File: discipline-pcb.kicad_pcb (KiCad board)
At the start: 2 copper layers, 357.2 x 120.3 mm, 160 parts, among them SW1 KEYSW, SW10 KEYSW, SW11 KEYSW, SW12 KEYSW, SW13 KEYSW, SW14 KEYSW, SW16 KEYSW, SW17 KEYSW, SW18 KEYSW, SW19 KEYSW, SW2 KEYSW, SW20 KEYSW, SW21 KEYSW, SW22 KEYSW, SW23 KEYSW, SW24 KEYSW, SW25 KEYSW, SW26 KEYSW, SW27 KEYSW, SW28 KEYSW, SW29 KEYSW, SW3 KEYSW, SW31 KEYSW, SW32 KEYSW, SW33 KEYSW, SW34 KEYSW, SW35 KEYSW, SW36 KEYSW, SW37 KEYSW, SW38 KEYSW, SW39 KEYSW, SW4 KEYSW, SW40 KEYSW, SW41 KEYSW, SW42 KEYSW, SW43 KEYSW, SW45 KEYSW, SW46 KEYSW, SW47 KEYSW, SW48 KEYSW, SW49 KEYSW, SW5 KEYSW, SW50 KEYSW, SW51 KEYSW, SW52 KEYSW, SW53 KEYSW, SW54 KEYSW, SW55 KEYSW, SW56 KEYSW, SW57 KEYSW, SW59 KEYSW, SW6 KEYSW, SW60 KEYSW, SW61 KEYSW, SW62 KEYSW, SW7 KEYSW, SW72 KEYSW, SW73 KEYSW, SW74 KEYSW, SW75 KEYSW, SW76 KEYSW, SW77 KEYSW, SW78 KEYSW, SW79 KEYSW, SW8 KEYSW, SW80 KEYSW, SW81 KEYSW, SW82 KEYSW, SW83 KEYSW, SW9 KEYSW

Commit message: update to hotswap; needs rerouting
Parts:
- removed ST62: 7U, cftkb:MX-7U-Stabilizer
- SW1, SW10, SW11, SW12, SW13, SW17, SW18, SW19, SW2, SW20, SW21, SW22, SW23, SW24, SW25, SW26, SW27, SW28, SW3, SW32, SW33, SW34, SW35, SW36, SW37, SW38, SW39, SW4, SW40, SW41, SW42, SW46, SW47, SW48, SW49, SW5, SW50, SW51, SW52, SW53, SW54, SW55, SW6, SW7, SW72, SW75, SW76, SW77, SW78, SW79, SW8, SW80, SW81, SW82, SW83, SW9: footprint cftkb:SW_Cherry_MX1A_1.00u_PCB-NOSCREEN -> MX_Hotswap:MX-Hotswap-1U; moved to B.Cu
- SW14: footprint cftkb:SW_Cherry_MX1A_2.00u_PCBNOSCREEN -> MX_Hotswap:MX-Hotswap-2U; moved to B.Cu
- SW16, SW29, SW73, SW74: footprint cftkb:SW_Cherry_MX1A_1.50u_PCBNOSCREEN -> MX_Hotswap:MX-Hotswap-1.5U; moved to B.Cu
- SW31: footprint cftkb:SW_Cherry_MX1A_1.75u_PCBNOSCREEN -> MX_Hotswap:MX-Hotswap-1.75U; moved to B.Cu
- SW43, SW45: footprint cftkb:SW_Cherry_MX1A_2.25u_PCBNOSCREEN -> MX_Hotswap:MX-Hotswap-2.25U; moved to B.Cu
- SW56: footprint cftkb:SW_Cherry_MX1A_2.75u_PCB_NOSCREEN -> MX_Hotswap:MX-Hotswap-2.75U; moved to B.Cu
- SW57, SW59, SW60, SW61: footprint cftkb:SW_Cherry_MX1A_1.25u_PCBNOSCREEN -> MX_Hotswap:MX-Hotswap-1.25U; moved to B.Cu
- SW62: footprint cftkb:SW_Cherry_MX1A_1.00u_PCB-NOSCREEN -> MX_Hotswap:MX-Hotswap-7U-ReversedStabilizers; moved to B.Cu
- moved ? 20.6 mm to (399.5, 104.5)
- moved SW10 5.68 mm to (234.8, 94.8), turned to 180 degrees
- moved SW11 5.68 mm to (253.8, 94.8), turned to 180 degrees
- moved SW5 5.68 mm to (139.5, 94.8), turned to 180 degrees
- moved SW50 5.68 mm to (182.4, 151.9), turned to 180 degrees
- moved SW54 5.68 mm to (258.6, 151.9), turned to 180 degrees
- moved SW55 5.68 mm to (277.7, 151.9), turned to 180 degrees
- moved SW56 5.68 mm to (313.4, 151.9), turned to 180 degrees
- moved SW75 5.68 mm to (382.4, 94.8), turned to 180 degrees
- moved SW77 5.68 mm to (382.4, 151.9), turned to 180 degrees
- moved SW79 5.68 mm to (401.5, 94.8), turned to 180 degrees
- moved SW2 5.68 mm to (82.4, 94.8), turned to 180 degrees
- moved SW3 5.68 mm to (101.4, 94.8), turned to 180 degrees
- moved SW4 5.68 mm to (120.5, 94.8), turned to 180 degrees
- moved SW45 5.68 mm to (75.2, 151.9), turned to 180 degrees
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
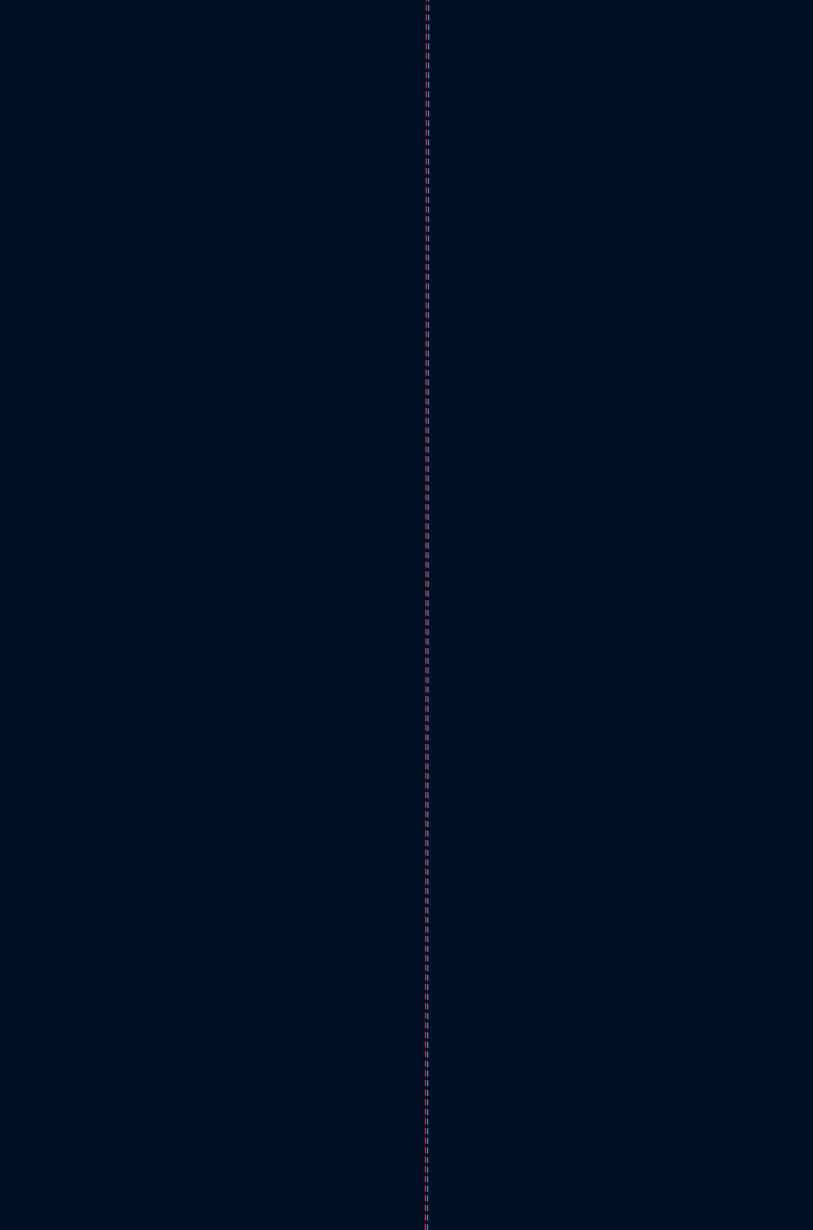
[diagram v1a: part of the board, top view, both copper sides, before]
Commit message: add leds to pcb
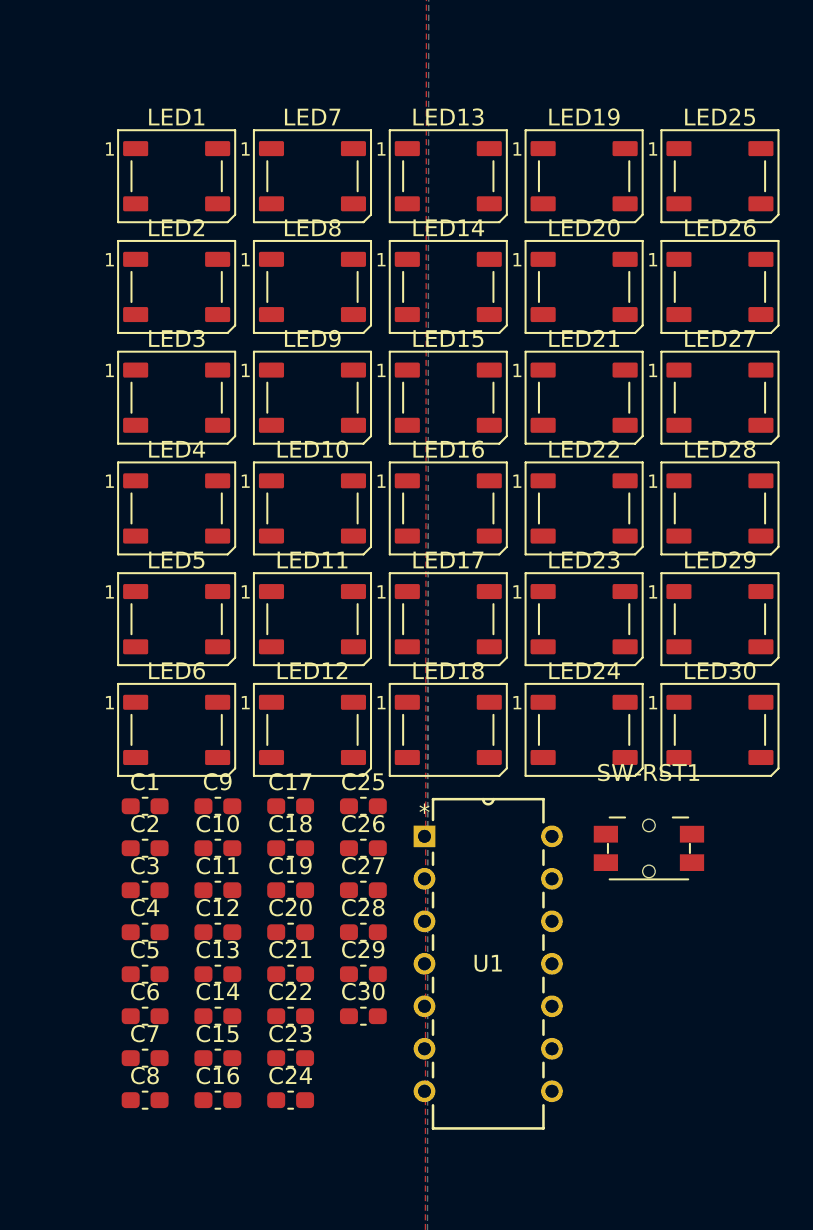
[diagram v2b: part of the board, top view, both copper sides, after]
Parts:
- added C1: 100nF 0603, Capacitor_SMD:C_0603_1608Metric_Pad1.08x0.95mm_HandSolder, F.Cu at (445.2, 128.2)
- added C10: 100nF 0603, Capacitor_SMD:C_0603_1608Metric_Pad1.08x0.95mm_HandSolder, F.Cu at (449.5, 130.7)
- added C11: 100nF 0603, Capacitor_SMD:C_0603_1608Metric_Pad1.08x0.95mm_HandSolder, F.Cu at (449.5, 133.2)
- added C12: 100nF 0603, Capacitor_SMD:C_0603_1608Metric_Pad1.08x0.95mm_HandSolder, F.Cu at (449.5, 135.7)
- added C13: 100nF 0603, Capacitor_SMD:C_0603_1608Metric_Pad1.08x0.95mm_HandSolder, F.Cu at (449.5, 138.2)
- added C14: 100nF 0603, Capacitor_SMD:C_0603_1608Metric_Pad1.08x0.95mm_HandSolder, F.Cu at (449.5, 140.7)
- added C15: 100nF 0603, Capacitor_SMD:C_0603_1608Metric_Pad1.08x0.95mm_HandSolder, F.Cu at (449.5, 143.2)
- added C16: 100nF 0603, Capacitor_SMD:C_0603_1608Metric_Pad1.08x0.95mm_HandSolder, F.Cu at (449.5, 145.7)
- added C17: 100nF 0603, Capacitor_SMD:C_0603_1608Metric_Pad1.08x0.95mm_HandSolder, F.Cu at (453.9, 128.2)
- added C18: 100nF 0603, Capacitor_SMD:C_0603_1608Metric_Pad1.08x0.95mm_HandSolder, F.Cu at (453.9, 130.7)
- added C19: 100nF 0603, Capacitor_SMD:C_0603_1608Metric_Pad1.08x0.95mm_HandSolder, F.Cu at (453.9, 133.2)
- added C2: 100nF 0603, Capacitor_SMD:C_0603_1608Metric_Pad1.08x0.95mm_HandSolder, F.Cu at (445.2, 130.7)
- added C20: 100nF 0603, Capacitor_SMD:C_0603_1608Metric_Pad1.08x0.95mm_HandSolder, F.Cu at (453.9, 135.7)
- added C21: 100nF 0603, Capacitor_SMD:C_0603_1608Metric_Pad1.08x0.95mm_HandSolder, F.Cu at (453.9, 138.2)
- added C22: 100nF 0603, Capacitor_SMD:C_0603_1608Metric_Pad1.08x0.95mm_HandSolder, F.Cu at (453.9, 140.7)
- added C23: 100nF 0603, Capacitor_SMD:C_0603_1608Metric_Pad1.08x0.95mm_HandSolder, F.Cu at (453.9, 143.2)
- added C24: 100nF 0603, Capacitor_SMD:C_0603_1608Metric_Pad1.08x0.95mm_HandSolder, F.Cu at (453.9, 145.7)
- added C25: 100nF 0603, Capacitor_SMD:C_0603_1608Metric_Pad1.08x0.95mm_HandSolder, F.Cu at (458.2, 128.2)
- added C26: 100nF 0603, Capacitor_SMD:C_0603_1608Metric_Pad1.08x0.95mm_HandSolder, F.Cu at (458.2, 130.7)
- added C27: 100nF 0603, Capacitor_SMD:C_0603_1608Metric_Pad1.08x0.95mm_HandSolder, F.Cu at (458.2, 133.2)
- added C28: 100nF 0603, Capacitor_SMD:C_0603_1608Metric_Pad1.08x0.95mm_HandSolder, F.Cu at (458.2, 135.7)
- added C29: 100nF 0603, Capacitor_SMD:C_0603_1608Metric_Pad1.08x0.95mm_HandSolder, F.Cu at (458.2, 138.2)
- added C3: 100nF 0603, Capacitor_SMD:C_0603_1608Metric_Pad1.08x0.95mm_HandSolder, F.Cu at (445.2, 133.2)
- added C30: 100nF 0603, Capacitor_SMD:C_0603_1608Metric_Pad1.08x0.95mm_HandSolder, F.Cu at (458.2, 140.7)
- added C4: 100nF 0603, Capacitor_SMD:C_0603_1608Metric_Pad1.08x0.95mm_HandSolder, F.Cu at (445.2, 135.7)
- added C5: 100nF 0603, Capacitor_SMD:C_0603_1608Metric_Pad1.08x0.95mm_HandSolder, F.Cu at (445.2, 138.2)
- added C6: 100nF 0603, Capacitor_SMD:C_0603_1608Metric_Pad1.08x0.95mm_HandSolder, F.Cu at (445.2, 140.7)
- added C7: 100nF 0603, Capacitor_SMD:C_0603_1608Metric_Pad1.08x0.95mm_HandSolder, F.Cu at (445.2, 143.2)
- added C8: 100nF 0603, Capacitor_SMD:C_0603_1608Metric_Pad1.08x0.95mm_HandSolder, F.Cu at (445.2, 145.7)
- added C9: 100nF 0603, Capacitor_SMD:C_0603_1608Metric_Pad1.08x0.95mm_HandSolder, F.Cu at (449.5, 128.2)
- added LED1: WS2812B, LED_SMD:LED_WS2812B_PLCC4_5.0x5.0mm_P3.2mm, F.Cu at (447.1, 90.5)
- added LED10: WS2812B, LED_SMD:LED_WS2812B_PLCC4_5.0x5.0mm_P3.2mm, F.Cu at (455.2, 110.4)
- added LED11: WS2812B, LED_SMD:LED_WS2812B_PLCC4_5.0x5.0mm_P3.2mm, F.Cu at (455.2, 117.0)
- added LED12: WS2812B, LED_SMD:LED_WS2812B_PLCC4_5.0x5.0mm_P3.2mm, F.Cu at (455.2, 123.6)
- added LED13: WS2812B, LED_SMD:LED_WS2812B_PLCC4_5.0x5.0mm_P3.2mm, F.Cu at (463.3, 90.5)
- added LED14: WS2812B, LED_SMD:LED_WS2812B_PLCC4_5.0x5.0mm_P3.2mm, F.Cu at (463.3, 97.1)
- added LED15: WS2812B, LED_SMD:LED_WS2812B_PLCC4_5.0x5.0mm_P3.2mm, F.Cu at (463.3, 103.7)
- added LED16: WS2812B, LED_SMD:LED_WS2812B_PLCC4_5.0x5.0mm_P3.2mm, F.Cu at (463.3, 110.4)
- added LED17: WS2812B, LED_SMD:LED_WS2812B_PLCC4_5.0x5.0mm_P3.2mm, F.Cu at (463.3, 117.0)
- added LED18: WS2812B, LED_SMD:LED_WS2812B_PLCC4_5.0x5.0mm_P3.2mm, F.Cu at (463.3, 123.6)
- added LED19: WS2812B, LED_SMD:LED_WS2812B_PLCC4_5.0x5.0mm_P3.2mm, F.Cu at (471.4, 90.5)
- added LED2: WS2812B, LED_SMD:LED_WS2812B_PLCC4_5.0x5.0mm_P3.2mm, F.Cu at (447.1, 97.1)
- added LED20: WS2812B, LED_SMD:LED_WS2812B_PLCC4_5.0x5.0mm_P3.2mm, F.Cu at (471.4, 97.1)
- added LED21: WS2812B, LED_SMD:LED_WS2812B_PLCC4_5.0x5.0mm_P3.2mm, F.Cu at (471.4, 103.7)
- added LED22: WS2812B, LED_SMD:LED_WS2812B_PLCC4_5.0x5.0mm_P3.2mm, F.Cu at (471.4, 110.4)
- added LED23: WS2812B, LED_SMD:LED_WS2812B_PLCC4_5.0x5.0mm_P3.2mm, F.Cu at (471.4, 117.0)
- added LED24: WS2812B, LED_SMD:LED_WS2812B_PLCC4_5.0x5.0mm_P3.2mm, F.Cu at (471.4, 123.6)
- added LED25: WS2812B, LED_SMD:LED_WS2812B_PLCC4_5.0x5.0mm_P3.2mm, F.Cu at (479.6, 90.5)
- added LED26: WS2812B, LED_SMD:LED_WS2812B_PLCC4_5.0x5.0mm_P3.2mm, F.Cu at (479.6, 97.1)
- added LED27: WS2812B, LED_SMD:LED_WS2812B_PLCC4_5.0x5.0mm_P3.2mm, F.Cu at (479.6, 103.7)
- added LED28: WS2812B, LED_SMD:LED_WS2812B_PLCC4_5.0x5.0mm_P3.2mm, F.Cu at (479.6, 110.4)
- added LED29: WS2812B, LED_SMD:LED_WS2812B_PLCC4_5.0x5.0mm_P3.2mm, F.Cu at (479.6, 117.0)
- added LED3: WS2812B, LED_SMD:LED_WS2812B_PLCC4_5.0x5.0mm_P3.2mm, F.Cu at (447.1, 103.7)
- added LED30: WS2812B, LED_SMD:LED_WS2812B_PLCC4_5.0x5.0mm_P3.2mm, F.Cu at (479.6, 123.6)
- added LED4: WS2812B, LED_SMD:LED_WS2812B_PLCC4_5.0x5.0mm_P3.2mm, F.Cu at (447.1, 110.4)
- added LED5: WS2812B, LED_SMD:LED_WS2812B_PLCC4_5.0x5.0mm_P3.2mm, F.Cu at (447.1, 117.0)
- added LED6: WS2812B, LED_SMD:LED_WS2812B_PLCC4_5.0x5.0mm_P3.2mm, F.Cu at (447.1, 123.6)
- added LED7: WS2812B, LED_SMD:LED_WS2812B_PLCC4_5.0x5.0mm_P3.2mm, F.Cu at (455.2, 90.5)
- added LED8: WS2812B, LED_SMD:LED_WS2812B_PLCC4_5.0x5.0mm_P3.2mm, F.Cu at (455.2, 97.1)
- added LED9: WS2812B, LED_SMD:LED_WS2812B_PLCC4_5.0x5.0mm_P3.2mm, F.Cu at (455.2, 103.7)
- added SW-RST1: EVQ, Button_Switch_SMD:Panasonic_EVQPUM_EVQPUD, F.Cu at (475.3, 130.7)
- added U1: SN74AHCT125N, footprints:N14, F.Cu at (469.5, 145.2)
- renumbered LED1 to LED_5V1
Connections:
- A1 pad 22: unconnected-(A1-GPIO17-Pad22) -> ledpin
- A1 pad 30: unconnected-(A1-RUN-Pad30) -> Resetbtn
- A1 pad 39: unconnected-(A1-VSYS-Pad39) -> VSYS
